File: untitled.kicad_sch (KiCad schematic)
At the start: 23 parts, among them U5 RP2040, U6 W25Q128JVS, U7 E22-900M30S, Y1 ABM8-272-T3

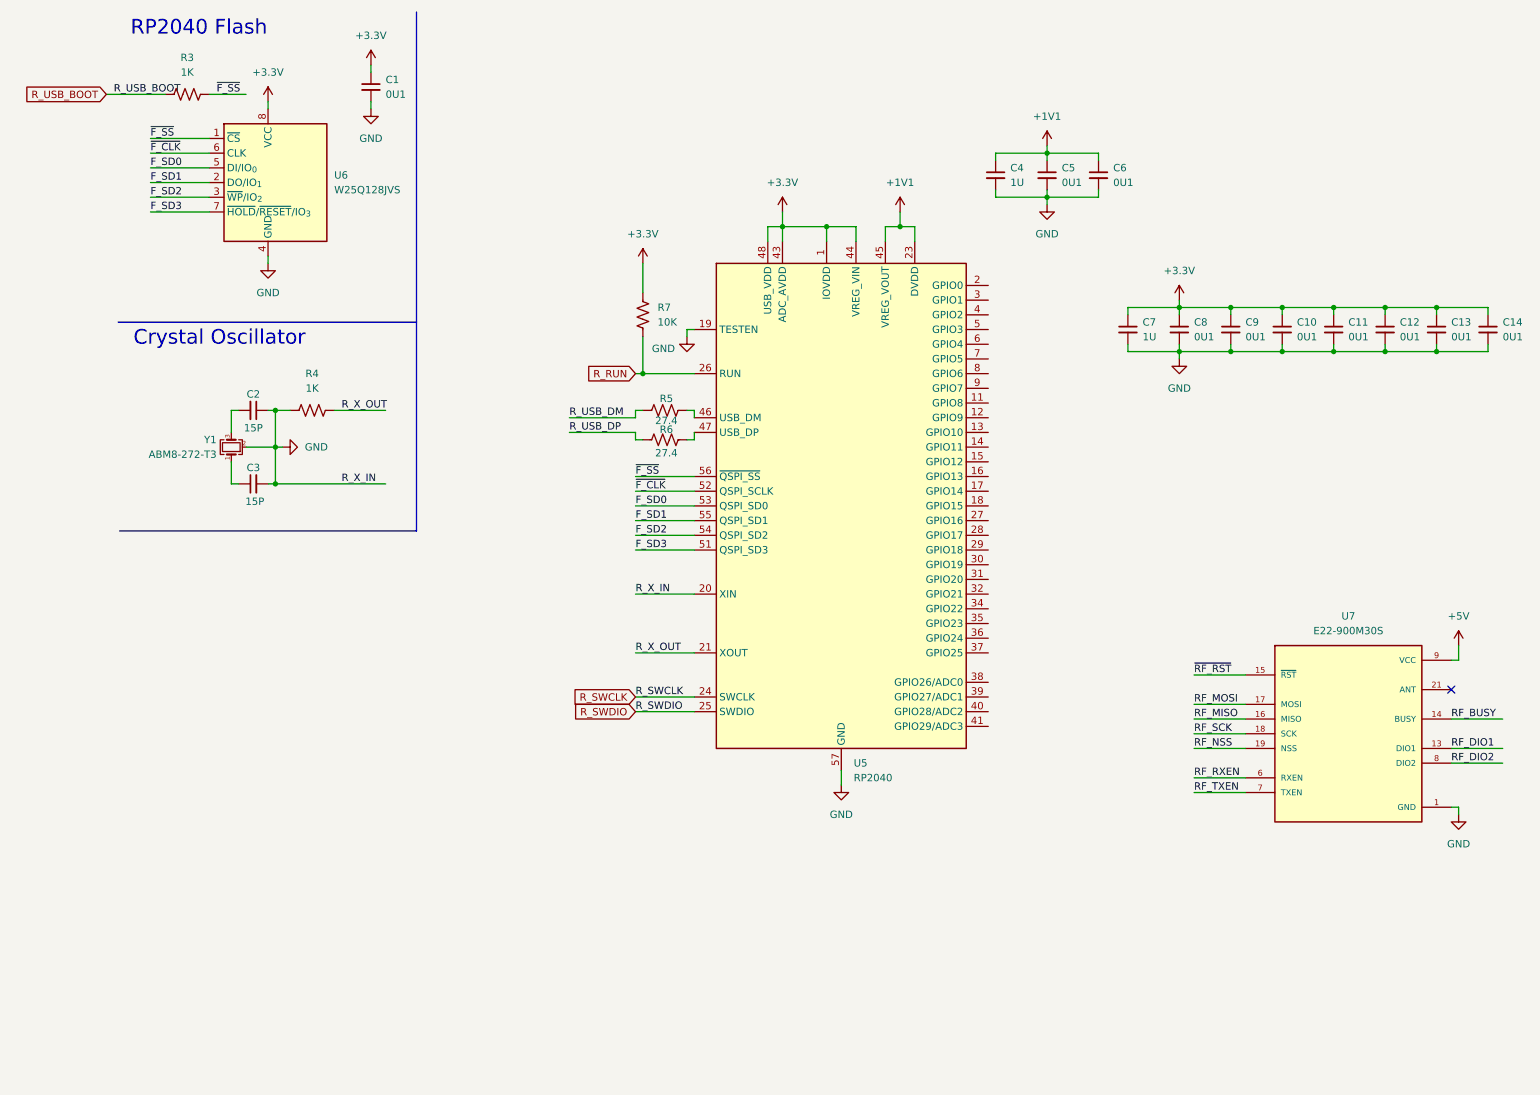
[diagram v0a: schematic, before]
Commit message: place all components
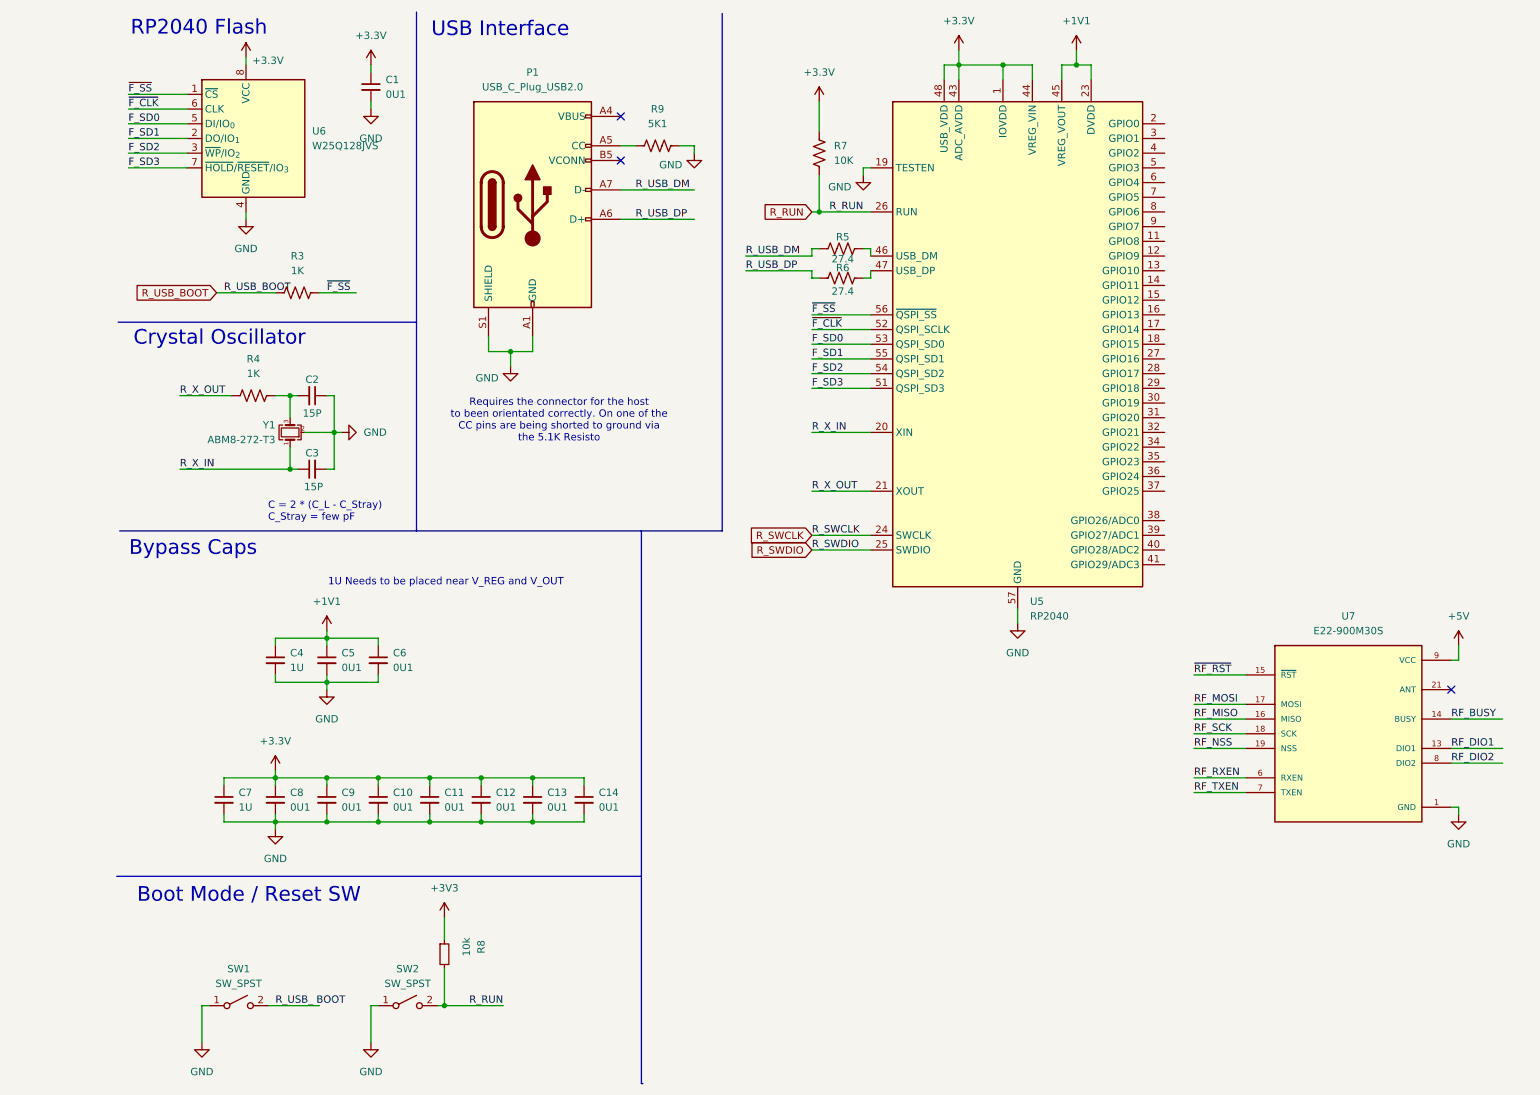
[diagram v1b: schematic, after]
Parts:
- added P1: USB_C_Plug_USB2.0, Connector_USB:USB_C_Receptacle_GCT_USB4110, symbol Connector:USB_C_Plug_USB2.0
- added R8: 10k, Resistor_SMD:R_0402_1005Metric, symbol Device:R_Small
- added R9: 5K1, Resistor_SMD:R_0603_1608Metric, symbol Device:R_US
- added SW1, SW2: SW_SPST, Button_Switch_SMD:SW_Push_1P1T_NO_CK_KMR2, symbol Switch:SW_SPST
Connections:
- net GND: now also P1.A1 (GND), P1.A12 (GND), P1.B1 (GND), P1.B12 (GND), P1.S1 (SHIELD), R9.2, SW1.1 (A), SW2.1 (A); no longer R4.1, U5.20 (XIN)
- net R_RUN: now also R8.2, SW2.2 (B)
- net R_USB_DM: now also P1.A7 (D-)
- net R_USB_DP: now also P1.A6 (D+)
- net R_X_OUT: now also R4.1; no longer R4.2
- net at C2.2, Y1.3: now also R4.2
- net R_X_IN: now reaches C3.1, Y1.1
- net R_X_IN: now also U5.20 (XIN)
- new net: P1.A4 (VBUS), P1.A9 (VBUS), P1.B4 (VBUS), P1.B9 (VBUS)
- new net: P1.A5 (CC), R9.1
- new net +3V3: R8.1
- new net R_USB_ BOOT: SW1.2 (B)
- no-connect marks 1 -> 3
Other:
- note added: "1U Needs to be placed near V_REG and V_OUT"
- note added: "Boot Mode / Reset SW"
- note added: "Bypass Caps"
- note added: "C = 2 * (C_L - C_Stray) C_Stray = few pF"
- note added: "Requires the connector for the host to been orientated correctly. On one of the CC pins are being shorted to ground via the 5.1K Resisto"
- note added: "USB Interface"
- moved on the sheet: C10, C11, C12, C13, C14, C2, C3, C4, C5, C6, C7, C8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
